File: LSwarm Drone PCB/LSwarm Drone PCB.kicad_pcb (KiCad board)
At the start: 4 copper layers, 100 x 99.8 mm, 134 parts, among them J2 Conn_01x06_Pin, J3 JST / BT2.0 Connector, J4 Conn_01x02_Pin, J5 Conn_01x02_Pin, J6 Conn_01x02_Pin, J7 Conn_01x02_Pin, J8 Conn_01x05_Pin, Q1 AO3400A, Q2 AO3400A, Q3 AO3400A, Q4 AO3400A, Q7 AO3407A, SW1 MSK12C02, SW2 SKRPACE010, SW3 SKRPACE010, SW4 SKRPACE010, SW5 SKRPACE010, U1 LSM6DSRTR, U12 AP2112K-3.3, U3 TPS61023DRLR, U4 SN74LVC1T45DBVR, U5 BMP581, X1 X322512MSB4SI

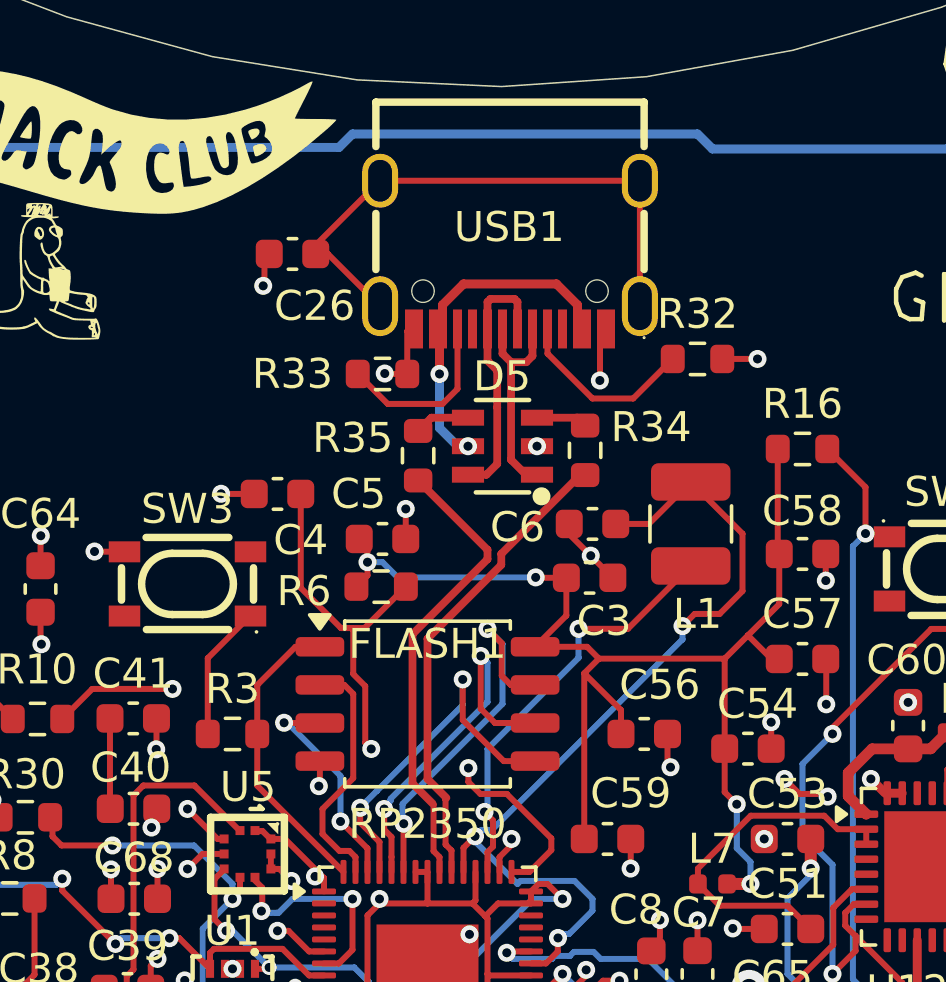
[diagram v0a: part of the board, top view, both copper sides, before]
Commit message: sync
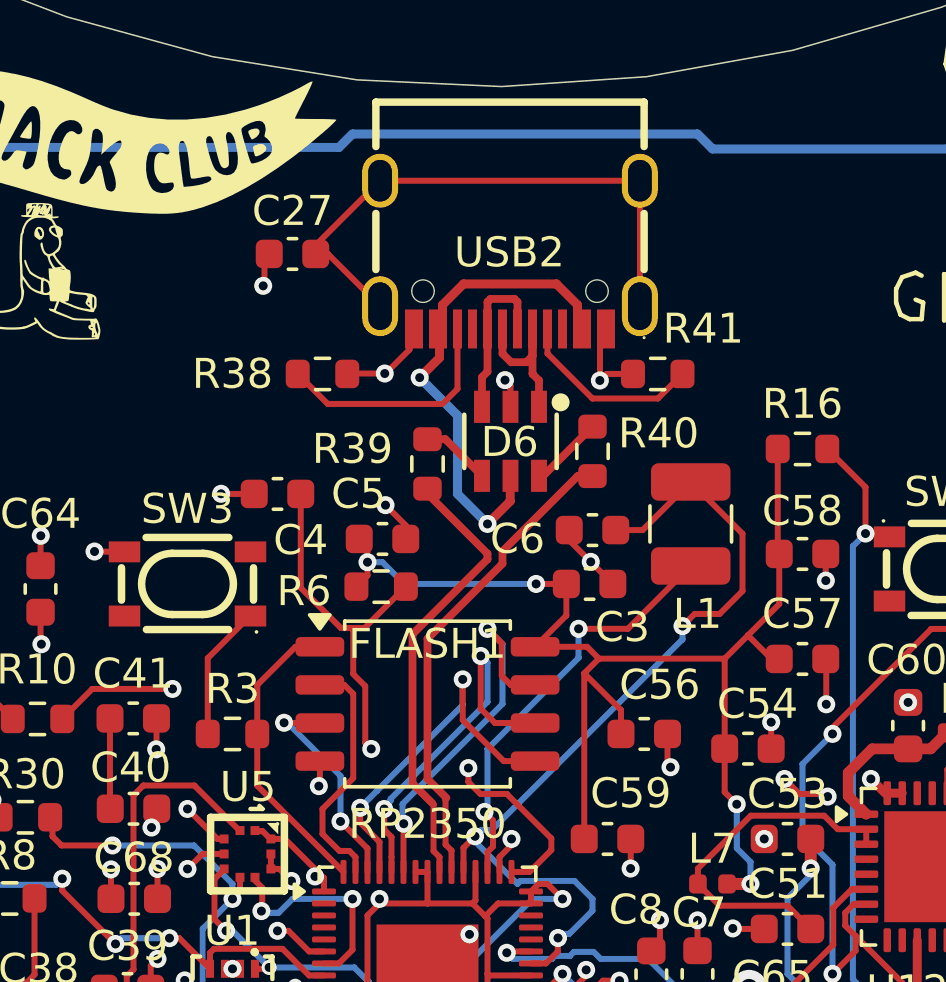
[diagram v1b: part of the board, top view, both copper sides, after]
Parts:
- removed C26: 10nF, Capacitor_SMD:C_0603_1608Metric
- removed D5: USBLC6-2SC6_C2687116, easyeda2kicad:SOT-23-6_L2.9-W1.6-P0.95-LS2.8-BL
- removed R32, R33: 5.1k, Resistor_SMD:R_0603_1608Metric
- removed R34, R35: 27, Resistor_SMD:R_0603_1608Metric
- removed USB1: USB-TYPE-C-018, easyeda2kicad:USB-C_SMD-TYPE-C-31-M-12
- added C27: 10nF, Capacitor_SMD:C_0603_1608Metric, F.Cu at (43.0, 25.0)
- added D6: USBLC6-2SC6_C2687116, easyeda2kicad:SOT-23-6_L2.9-W1.6-P0.95-LS2.8-BL, F.Cu at (50.3, 31.2)
- added R38: 5.1k, Resistor_SMD:R_0603_1608Metric, F.Cu at (44.0, 29.0)
- added R39: 27, Resistor_SMD:R_0603_1608Metric, F.Cu at (47.5, 32.0)
- added R40: 27, Resistor_SMD:R_0603_1608Metric, F.Cu at (53.0, 31.6)
- added R41: 5.1k, Resistor_SMD:R_0603_1608Metric, F.Cu at (55.2, 29.0)
- added USB2: USB-TYPE-C-018, easyeda2kicad:USB-C_SMD-TYPE-C-31-M-12, F.Cu at (50.2, 25.0)
- moved C3 0.21 mm to (52.9, 36.0)
- moved C6 0.21 mm to (53.0, 34.2)
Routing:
- net Net-(C27-Pad2): track 0.00 -> 19.3 mm
- net Net-(C26-Pad2): track 19.3 -> 0.00 mm
- net USB_VBUS: track 0.00 -> 15.9 mm, vias 0 -> 2
- net Net-(D5-VBUS): track 11.2 -> 0.00 mm, vias 2 -> 0
- net Net-(USB2-CC2): track 0.00 -> 7.95 mm
- net Net-(USB2-CC1): track 0.00 -> 6.28 mm
- net Net-(USB1-CC1): track 6.16 -> 0.00 mm
- net Net-(USB1-CC2): track 5.95 -> 0.00 mm
- net USB_D+: track 8.64 -> 5.55 mm
- net GND: track 132.4 -> 134.9 mm, vias 99 -> 98
- net Net-(D6-I/O1-Pad6): track 0.00 -> 2.46 mm
- net Net-(D6-I/O2-Pad4): track 0.00 -> 2.44 mm
- net Net-(D5-I/O2-Pad4): track 1.85 -> 0.00 mm
- net Net-(D5-I/O2-Pad3): track 1.71 -> 0.00 mm
- net USB_D-: track 7.25 -> 5.61 mm
